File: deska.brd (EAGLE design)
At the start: 100 x 80 mm, 12 parts, among them IC1 78L05Z, T1 TIP122, T2 TIP122, T3 TIP122

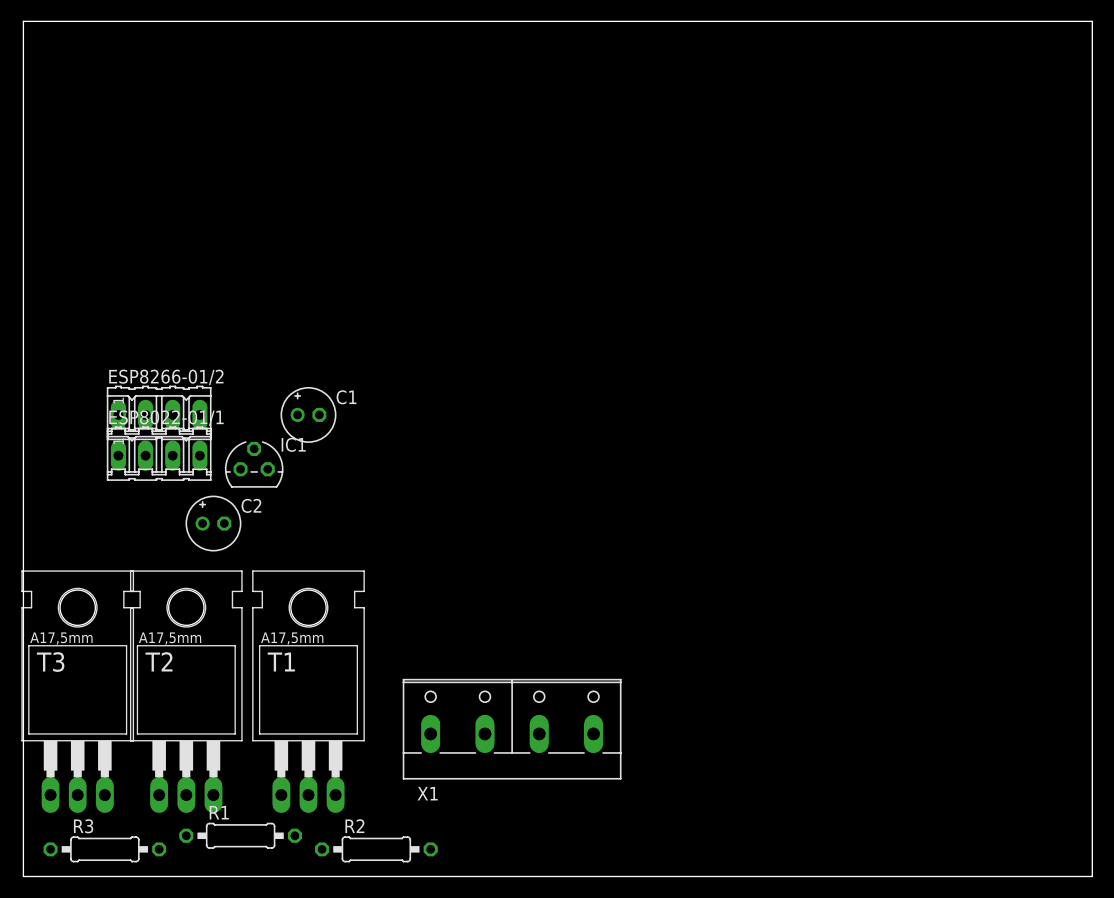
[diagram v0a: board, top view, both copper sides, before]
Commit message: zmeny plosnaku
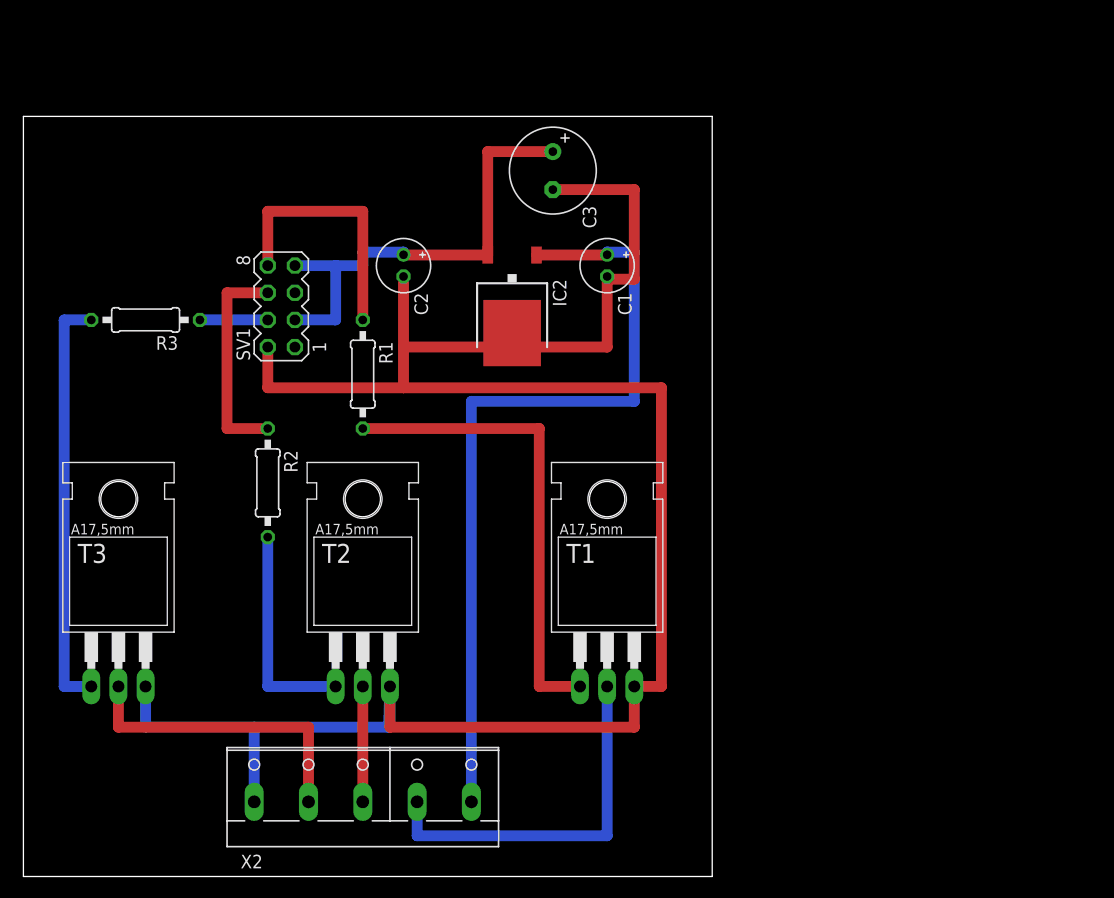
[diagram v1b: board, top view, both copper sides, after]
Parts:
- removed ESP8022-01/1, ESP8266-01/2: (no value), con-amp-quick:04P
- removed IC1: 78L05Z, linear:TO92
- removed X1: (no value), con-wago-508:W237-4P
- added C3: 220u, rcl:E3,5-8
- added IC2: LF33CDT, linear:TO252
- added SV1: ESP8266, con-lstb:MA04-2
- added X2: NAPAJENI, con-wago-508:W237-5P
- C1: value (none) -> 0,1u
- C2: value (none) -> 2.2u
- R1, R2, R3: value (none) -> 1k
- moved R3 49.7 mm to (11.4, 52.1), turned to 180 degrees
- moved R1 44.7 mm to (31.8, 47.0), turned to 270 degrees
- moved R2 35.8 mm to (22.9, 36.8), turned to 270 degrees
- moved C1 31.2 mm to (54.6, 57.1), turned to 270 degrees
- moved C2 30.0 mm to (35.6, 57.1), turned to 270 degrees
- moved T1 29.7 mm to (54.6, 24.1)
- moved T2 19.4 mm to (31.8, 24.1)
- moved T3 10.9 mm to (8.89, 24.1)
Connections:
- net +12V: now also IC2.1, X2.5; no longer IC1.3, X1.4
- net GND: now also C3.-, IC2.3, SV1.2, X2.1; no longer ESP8266-01/2.4, IC1.2
- net N$1: now also X2.4; no longer X1.3
- net N$10: now also SV1.4; no longer ESP8266-01/2.3
- net N$11: now also C3.+, IC2.2, SV1.3, SV1.7; no longer ESP8022-01/1.2, ESP8022-01/1.3, ESP8022-01/1.4, IC1.1
- net N$2: now also X2.3; no longer X1.2
- net N$3: now also X2.2; no longer X1.1
- net N$7: now also SV1.8; no longer ESP8266-01/2.1
- net N$8: now also SV1.6; no longer ESP8266-01/2.2
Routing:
- net GND: track 0.00 -> 199.1 mm
- net +12V: track 0.00 -> 76.1 mm
- net N$4: track 0.00 -> 44.4 mm
- net N$11: track 0.00 -> 44.2 mm
- net N$6: track 0.00 -> 39.4 mm
- net N$1: track 0.00 -> 34.9 mm
- net N$3: track 0.00 -> 28.6 mm
- net N$7: track 0.00 -> 24.1 mm
- net N$8: track 0.00 -> 20.3 mm
- net N$5: track 0.00 -> 20.3 mm
- net N$2: track 0.00 -> 10.8 mm
- net N$10: track 0.00 -> 6.35 mm
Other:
- board size 100 x 80 mm -> 64.4 x 71.1 mm
